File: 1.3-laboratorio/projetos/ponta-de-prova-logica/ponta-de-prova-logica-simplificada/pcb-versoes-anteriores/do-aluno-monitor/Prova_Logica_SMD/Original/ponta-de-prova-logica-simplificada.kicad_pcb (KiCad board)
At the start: 2 copper layers, 21 parts, among them J1 Conn_01x02, J2 TEST_1P, J3 TEST_1P, SW1 SW_DPDT_x2, U1 LM339

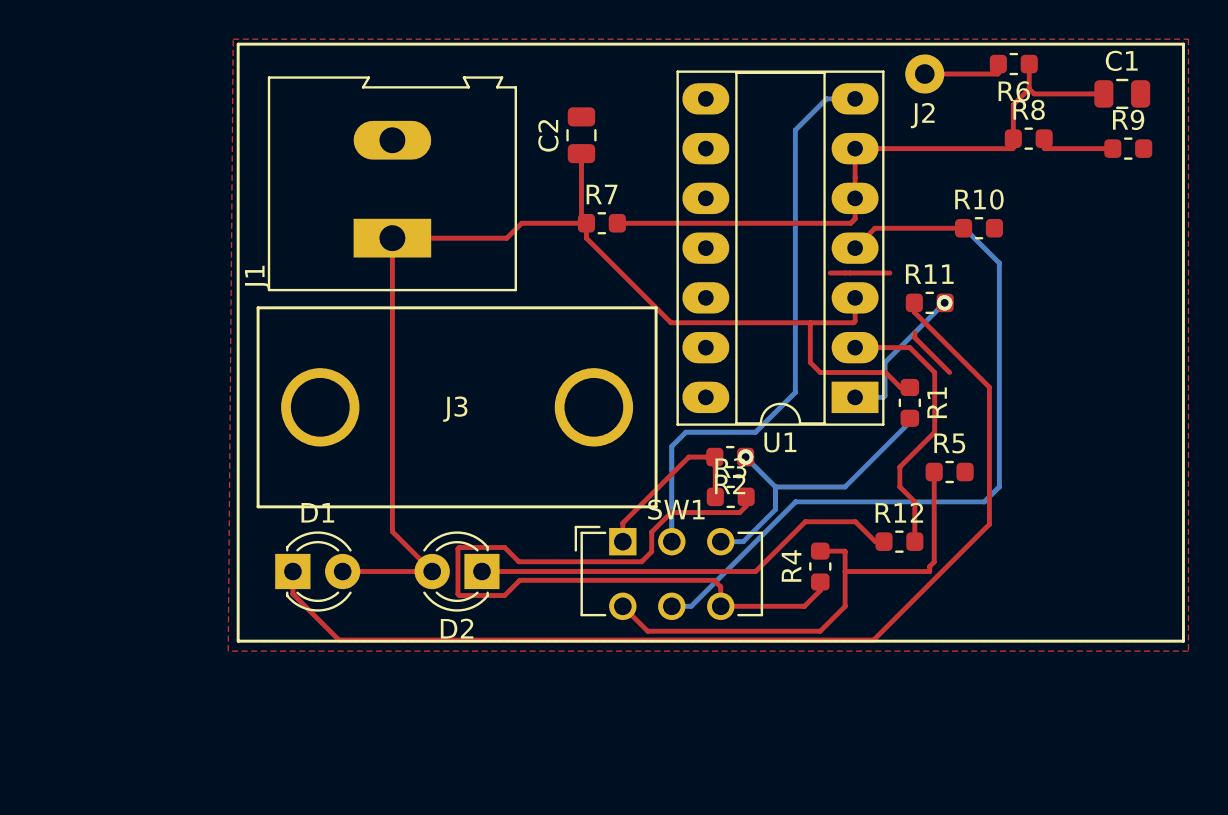
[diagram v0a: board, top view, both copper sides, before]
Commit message: Ponta_Logica_SMD_v2
Versao 2 - Projeto Ponta Lógica monitor
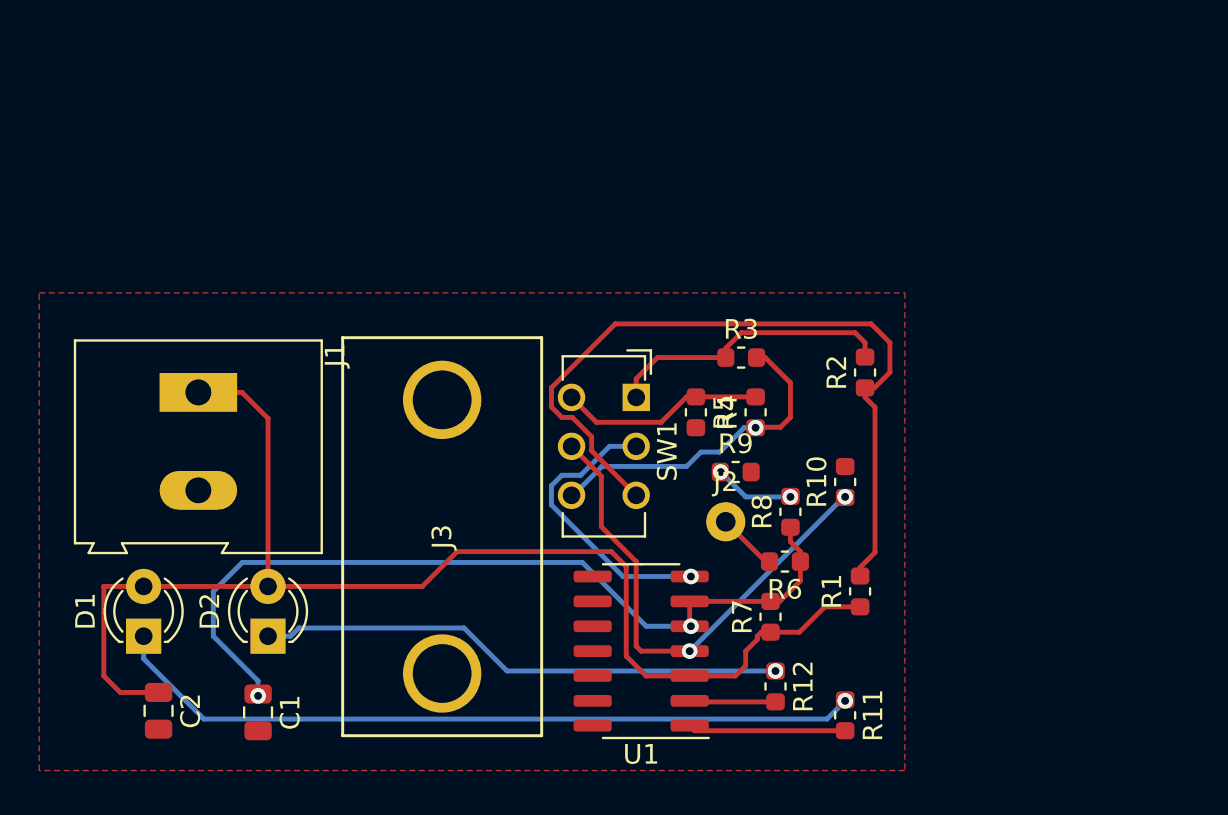
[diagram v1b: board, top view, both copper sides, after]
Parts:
- U1: footprint Package_DIP:DIP-14_W7.62mm_Socket_LongPads -> Package_SO:SOIC-14_3.9x8.7mm_P1.27mm
- moved C1 54.3 mm to (62.0, 184.7), turned to 270 degrees
- moved C2 36.5 mm to (56.9, 184.7), turned to 270 degrees
- moved R6 28.0 mm to (88.9, 177.0)
- moved R9 26.0 mm to (86.4, 172.5)
- moved J2 25.0 mm to (85.9, 175.0)
- moved R8 22.6 mm to (89.2, 174.5), turned to 90 degrees
- moved R7 21.9 mm to (88.1, 179.9), turned to 90 degrees
- moved R11 21.5 mm to (91.9, 184.9), turned to 270 degrees
- moved U1 16.9 mm to (81.5, 181.6)
- moved R10 14.6 mm to (91.9, 173.0), turned to 90 degrees
- moved R5 13.3 mm to (84.3, 169.4), turned to 270 degrees
- moved J1 12.7 mm to (58.9, 168.4), turned to 270 degrees
- moved D2 11.4 mm to (62.5, 180.8), turned to 90 degrees
- moved R1 9.96 mm to (92.7, 178.6), turned to 90 degrees
- moved R12 9.73 mm to (88.4, 183.4), turned to 270 degrees
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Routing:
- net Net-(R1-Pad2): track 15.0 -> 39.9 mm, vias 1 -> 0
- net Net-(R3-Pad2): track 40.3 -> 16.9 mm, vias 0 -> 2
- net Net-(R4-Pad2): track 26.0 -> 10.5 mm
- net Net-(SW1-Pad2): track 29.4 -> 14.8 mm, vias 0 -> 2
- net Net-(D1-Pad1): track 53.0 -> 38.6 mm, vias 0 -> 2
- net Net-(R10-Pad1): track 39.2 -> 25.6 mm, vias 0 -> 2
- net Net-(C1-Pad1): track 32.4 -> 42.9 mm, vias 0 -> 2
- net Net-(R12-Pad2): track 14.3 -> 4.40 mm
- net GND: track 5.82 -> 0.00 mm
- net VCC: track 61.6 -> 67.0 mm
- net Net-(R2-Pad2): track 9.56 -> 14.8 mm
- net Net-(D2-Pad1): track 22.0 -> 27.0 mm, vias 0 -> 2
- net Net-(J2-Pad1): track 4.25 -> 3.08 mm
- net Net-(R11-Pad2): track 7.57 -> 8.04 mm, vias 1 -> 0
- net Net-(R8-Pad2): track 3.99 -> 4.08 mm, vias 0 -> 2
